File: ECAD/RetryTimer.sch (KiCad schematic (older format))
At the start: 8 parts

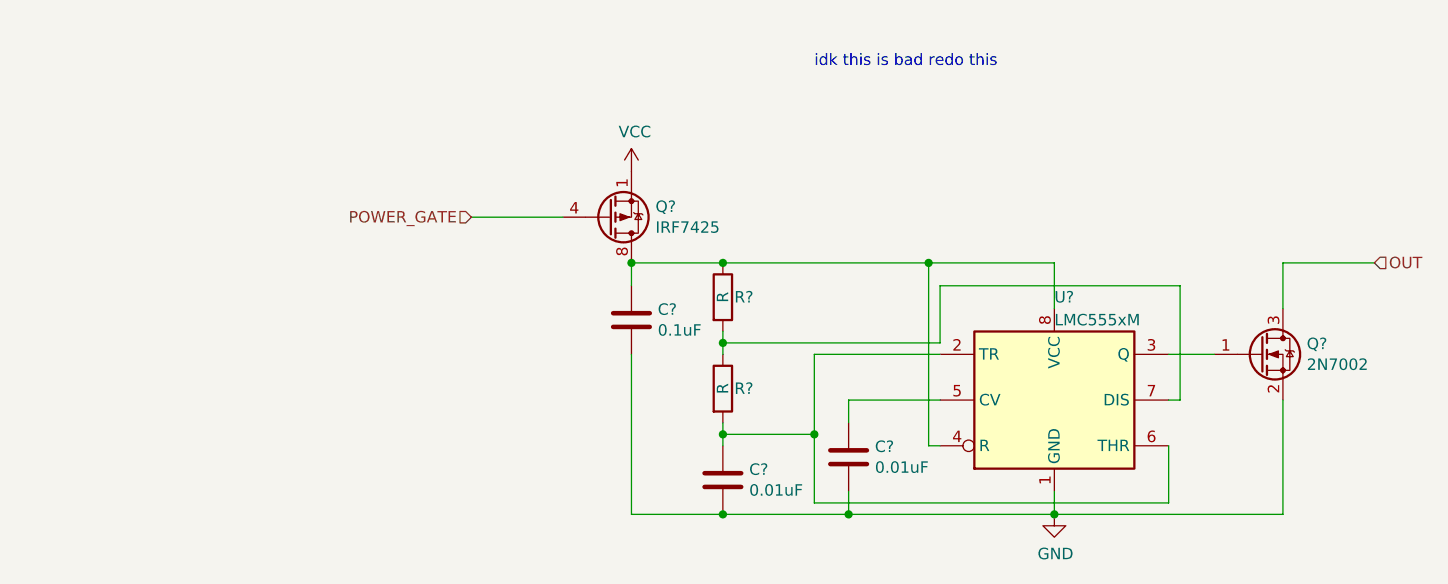
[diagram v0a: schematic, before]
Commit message: implement a retry timer
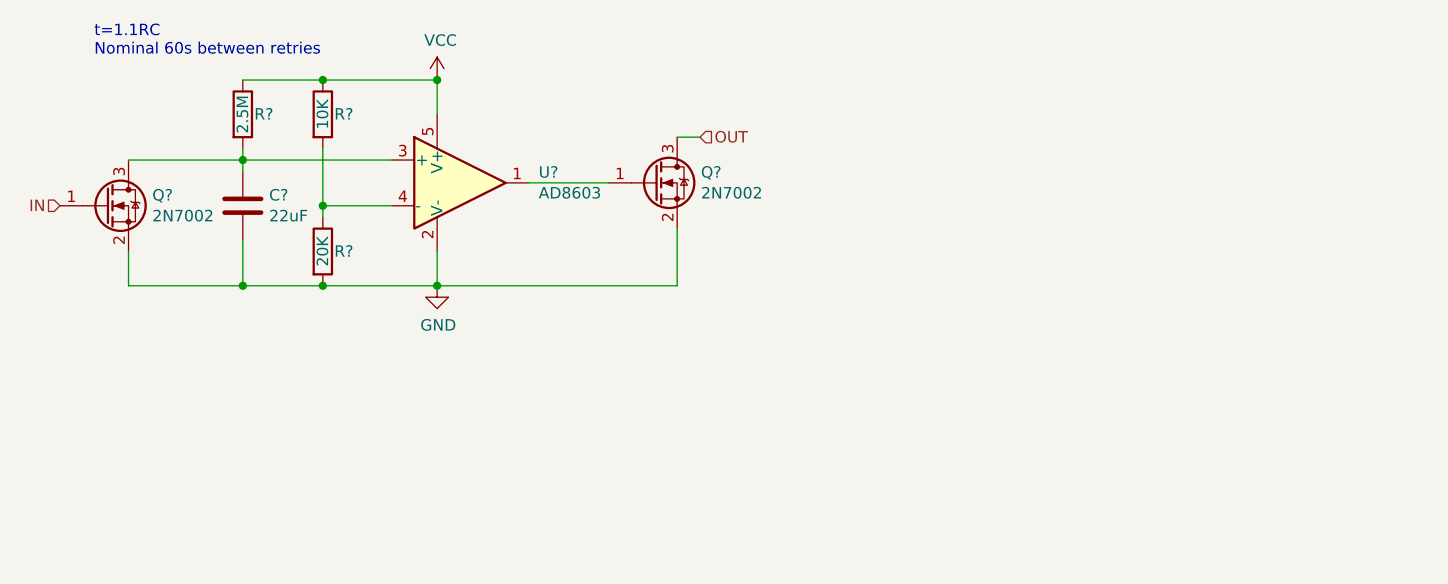
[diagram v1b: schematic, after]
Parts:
- removed C?: 0.01uF, symbol Device:C
- removed C?: 0.1uF, symbol Device:C
- removed Q?: IRF7425, Package_SO:SOIC-8_3.9x4.9mm_P1.27mm, symbol Transistor_FET:IRF7404
- removed Q?: 2N7002, Package_TO_SOT_SMD:SOT-23, symbol Transistor_FET:2N7002
- removed R?: R, symbol Device:R
- removed U?: LMC555xM, Package_SO:SOIC-8_3.9x4.9mm_P1.27mm, symbol Timer:LMC555xM
- added Q? (x2): 2N7002, Package_TO_SOT_SMD:SOT-23, symbol Transistor_FET:2N7002
- added R?: 10K, symbol Device:R
- added R?: 20K, symbol Device:R
- added U?: AD8603, Package_TO_SOT_SMD:TSOT-23-5, symbol Amplifier_Operational:AD8603
- C?: value 0.01uF -> 22uF
- R?: value R -> 2.5M
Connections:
- net GND: now also Q?.2 (S), Q?.2 (S), R?.2, U?.2 (V-)
- net OUT: now also Q?.3 (D)
- net VCC: now also R?.1, R?.1, U?.5 (V+)
- net at C?.1: now also R?.2, Q?.3 (D), U?.3 (+)
- new net: Q?.1 (G), U?.1
- new net: R?.1, R?.2, U?.4 (-)
- new net IN: Q?.1 (G)
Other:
- note added: "t=1.1RC\nNominal 60s between retries"
- note removed: "idk this is bad redo this"
- moved on the sheet: C?, R?
